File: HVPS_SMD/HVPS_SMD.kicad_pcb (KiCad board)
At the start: 2 copper layers, 36.8 x 22.9 mm, 22 parts, among them J1 CONN_01X02, J2 CONN_01X02, J3 CONN_01X02, Q1 AO4294, T1 MagTop-HVSMPS, U1 LM3478SOIC8

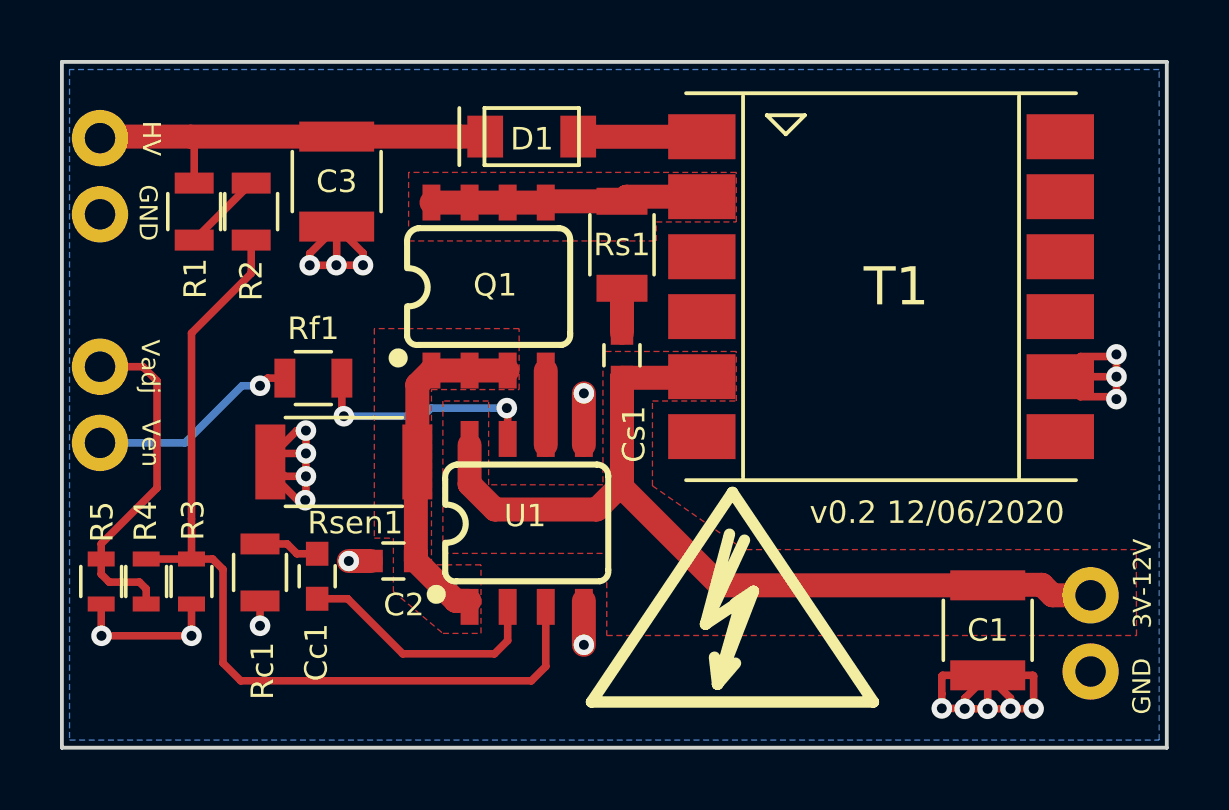
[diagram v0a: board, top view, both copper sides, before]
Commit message: Update Kicad6
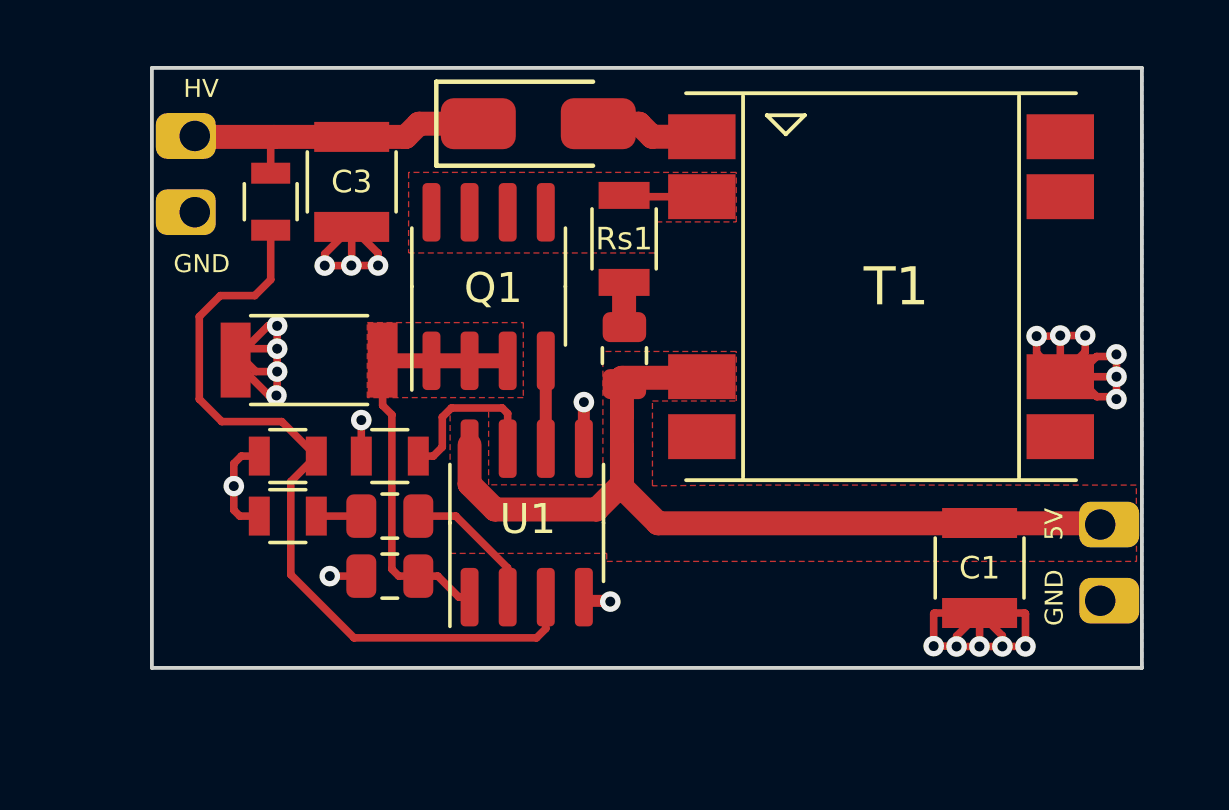
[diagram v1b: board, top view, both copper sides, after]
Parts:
- removed J3: CONN_01X02, lib_fp:SparkFun-Connectors-1X02_NO_SILK
- removed R2: 604k, lib_fp:R_0805
- removed R4, R5: 30k, lib_fp:R_0603
- removed REF**: Symbol_HighVoltage_Type2_CopperTop_VerySmall, logos:Symbol_HighVoltage_Type2_SilkTop_VerySmall
- removed Rsen1: 0.06, lib_fp:R_2010
- added Rs2: 0.062, lib_fp:R_2010, F.Cu at (187.3, 70.9)
- C2, Cc1, Cs1: footprint lib_fp:C_0603 -> Capacitor_SMD:C_0805_2012Metric
- D1: value ES1FL R3G -> ES1JF; footprint lib_fp:nixiemisc-DO-219AB -> NixieClockMaster:SMAF
- J1, J2: footprint lib_fp:SparkFun-Connectors-1X02_NO_SILK -> NixieClockMaster:Header_MA02-Edge
- Q1, U1: footprint lib_fp:nixiemisc-SO08 -> Package_SO:SOIC-8_3.9x4.9mm_P1.27mm
- R1: value 604k -> 10M
- R3: value 10.2k -> 69.8k; footprint lib_fp:R_0603 -> lib_fp:R_0805
- moved R3 5.27 mm to (186.6, 74.1), turned to 180 degrees
- moved J2 5.00 mm to (183.5, 62.2)
- moved Rf1 3.64 mm to (190.0, 74.1)
- moved Cc1 3.14 mm to (190.0, 76.1), turned to 180 degrees
- moved R1 2.57 mm to (186.0, 65.6)
- moved C1 2.09 mm to (209.7, 77.8)
- moved Rc1 2.09 mm to (186.6, 76.1), turned to 180 degrees
- moved J1 1.14 mm to (213.7, 80.2), turned to -90 degrees
- moved C2 0.52 mm to (190.0, 78.1)
- moved C3 0.50 mm to (188.7, 65.0)
- moved D1 0.48 mm to (194.9, 63.0)
- moved Rs1 0.21 mm to (197.8, 66.9)
- moved Cs1 0.08 mm to (197.8, 70.8)
- turned Q1 to 90 degrees
- turned U1 to 90 degrees
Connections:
- J1 pad 1: GND -> Vin
- J1 pad 2: Vin -> GND
- R3 pad 1: Net-(R2-Pad2) -> Net-(R1-Pad2)
- Rf1 pad 1: Ven -> GND
- T1 pad 1: Net-(D1-PadA) -> Net-(D1-Pad2)
- U1 pad 3: Net-(R2-Pad2) -> Net-(R1-Pad2)
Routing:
- net Net-(R2-Pad2): track 30.7 -> 0.00 mm
- net Net-(R1-Pad2): track 2.69 -> 26.8 mm
- net Vadj: track 11.5 -> 0.00 mm
- net Ven: track 7.06 -> 0.00 mm, vias 1 -> 0
- net Net-(Q1-Pad5): track 9.09 -> 2.55 mm
- net Net-(D1-PadA): track 4.12 -> 0.00 mm
- net Vout: track 14.7 -> 10.7 mm
- net Net-(Cc1-Pad1): track 8.62 -> 4.67 mm
- net Net-(D1-Pad2): track 0.00 -> 3.63 mm
- net Net-(C2-Pad1): track 11.4 -> 14.2 mm
- net Net-(Rf1-Pad2): track 7.88 -> 5.48 mm, vias 2 -> 0
- net GND: track 45.0 -> 47.2 mm, vias 21 -> 23
- net Vin: track 31.7 -> 30.7 mm
- net Net-(Cc1-Pad2): track 2.04 -> 1.50 mm
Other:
- board size 36.8 x 22.9 mm -> 33 x 20 mm
- net class 0.2mm removed
- net class Default removed
- net class Minimal removed
- board text added: "5V"
- board text removed: "3V-12V"
- board text removed: "Vadj"
- board text removed: "Ven"
- board text removed: "nixieclock.biz nixies.us hvps v0.2"
- board text removed: "v0.2 12/06/2020"
